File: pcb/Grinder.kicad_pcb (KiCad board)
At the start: 2 copper layers, 48 x 73 mm, 22 parts, among them J1 Conn_01x06, J2 Conn_01x05, J3 Conn_01x04, J4 Conn_02x05_Odd_Even, Q1 IRLZ44N, U1 ADS1232IPW

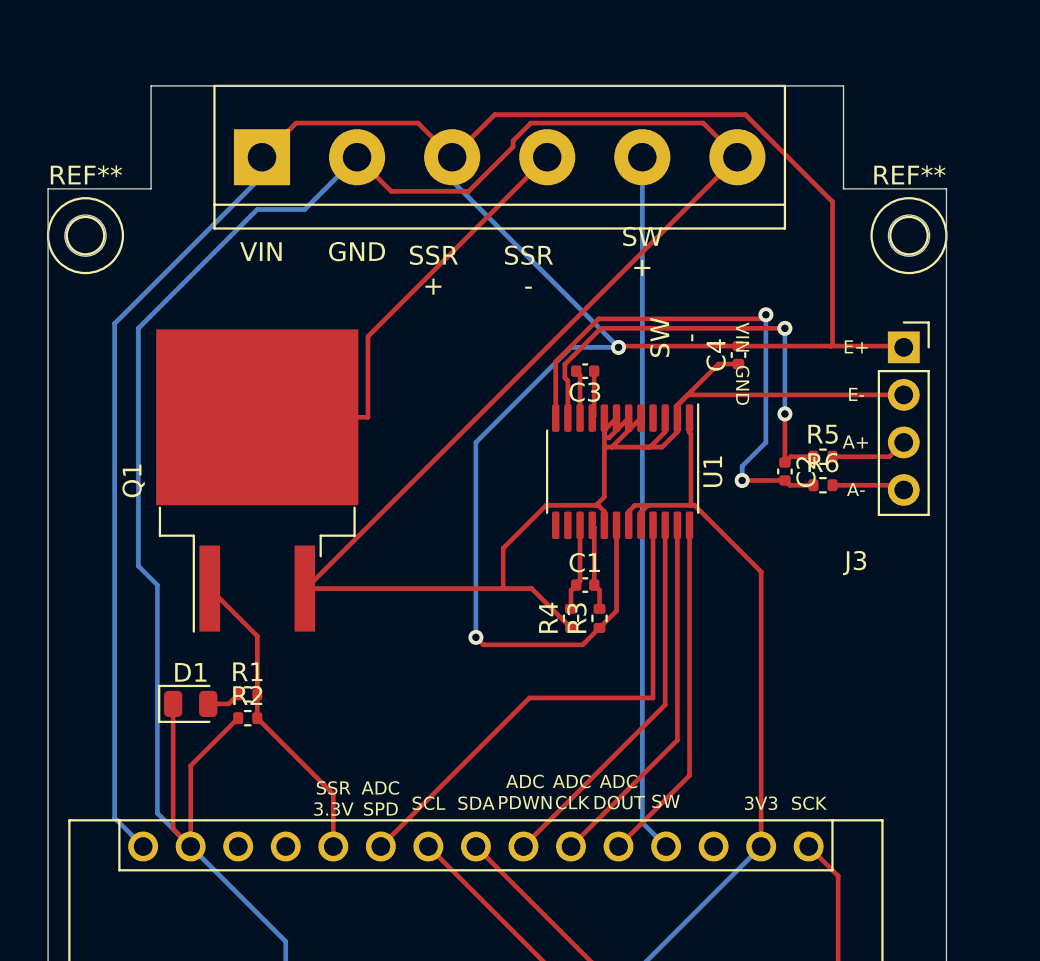
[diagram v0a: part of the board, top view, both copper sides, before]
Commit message: WIP
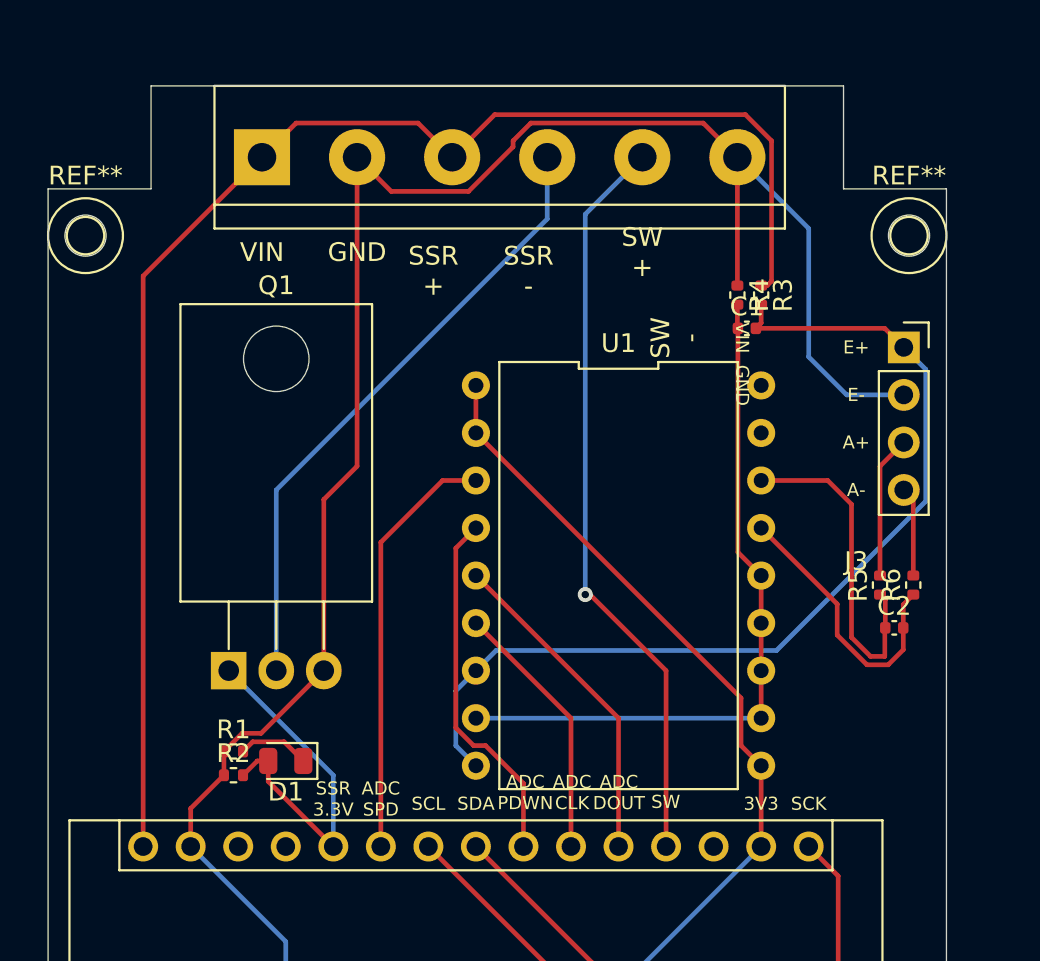
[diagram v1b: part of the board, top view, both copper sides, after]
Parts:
- removed C3: 100 nF, Capacitor_SMD:C_0402_1005Metric
- removed C4: 100nF, Capacitor_SMD:C_0402_1005Metric
- Q1: footprint Package_TO_SOT_SMD:TO-263-2 -> Package_TO_SOT_THT:TO-220-3_Horizontal_TabDown
- U1: value ADS1232IPW -> CJMCU-ADS1232; footprint Package_SO:TSSOP-24_4.4x7.8mm_P0.65mm -> custom:DIP-18_600
- moved R4 19.4 mm to (163.8, 55.6), turned to 270 degrees
- moved R3 19.3 mm to (165.1, 55.6), turned to 270 degrees
- moved C1 16.2 mm to (164.3, 57.4)
- moved Q1 10.3 mm to (136.7, 75.7), turned to 0 degrees
- moved C2 10.2 mm to (172.2, 73.4), turned to 0 degrees
- moved R5 7.50 mm to (171.4, 71.1), turned to 90 degrees
- moved R6 7.19 mm to (173.2, 71.1), turned to 90 degrees
- moved D1 5.92 mm to (139.7, 80.5), turned to 180 degrees
- moved U1 5.55 mm to (157.5, 70.6)
- moved R1 3.14 mm to (136.9, 80.0)
- moved R2 3.14 mm to (136.9, 81.3)
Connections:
- C2 pad 1: Net-(C2-Pad1) -> ADC_AINP1
- C2 pad 2: Net-(C2-Pad2) -> ADC_AINN1
- D1 pad 1: GND -> Net-(D1-Pad1)
- D1 pad 2: Net-(D1-Pad2) -> SSR_GATE
- J3 pad 1: 5V -> 5V_FILTERED
- R1 pad 1: Net-(D1-Pad2) -> GND
- R1 pad 2: SSR_GATE -> Net-(D1-Pad1)
- R5 pad 1: Net-(C2-Pad1) -> ADC_AINP1
- R6 pad 1: Net-(C2-Pad2) -> ADC_AINN1
- U1 pad 10: Net-(C3-Pad2) -> 3V3
- U1 pad 11: Net-(C2-Pad1) -> GNDA
- U1 pad 12: Net-(C2-Pad2) -> GNDA
- U1 pad 13: Net-(U1-Pad13) -> GNDA
- U1 pad 14: Net-(U1-Pad14) -> GNDA
- U1 pad 15: GNDA -> ADC_AINN1
- U1 pad 16: 5V_FILTERED -> ADC_AINP1
- U1 pad 17: GND -> Net-(U1-Pad17)
- U1 pad 18: 5V -> Net-(U1-Pad18)
- U1 pad 2: GND -> 3V3
- U1 pad 3: GND -> ADC_SPEED
- U1 pad 4: Net-(U1-Pad4) -> ADC_PDWN
- U1 pad 5: GND -> ADC_DOUT
- U1 pad 6: GND -> ADC_CLK
- U1 pad 7: GND -> 5V_FILTERED
- U1 pad 8: GND -> GNDA
- U1 pad 9: Net-(C3-Pad1) -> 5V_FILTERED
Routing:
- net GND: track 219.3 -> 133.6 mm
- net 5V: track 145.6 -> 80.2 mm, vias 2 -> 0
- net 5V_FILTERED: track 4.63 -> 52.2 mm
- net GNDA: track 4.66 -> 37.6 mm
- net Net-(C2-Pad2): track 28.6 -> 0.00 mm, vias 2 -> 0
- net Net-(C2-Pad1): track 24.3 -> 0.00 mm, vias 2 -> 0
- net ADC_AINP1: track 0.00 -> 18.1 mm
- net ADC_AINN1: track 0.00 -> 15.1 mm
- net SSR_DRAIN: track 23.8 -> 33.4 mm
- net ADC_CLK: track 19.5 -> 14.0 mm
- net ADC_SPEED: track 27.1 -> 22.7 mm
- net Net-(D1-Pad1): track 0.00 -> 3.86 mm
- net Net-(J3-Pad3): track 4.12 -> 7.64 mm
- net SSR_GATE: track 16.5 -> 19.4 mm
- net MANUAL_SW: track 37.4 -> 40.0 mm, vias 0 -> 1
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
